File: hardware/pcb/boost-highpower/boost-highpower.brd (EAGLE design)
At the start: 41.1 x 22.3 mm, 28 parts

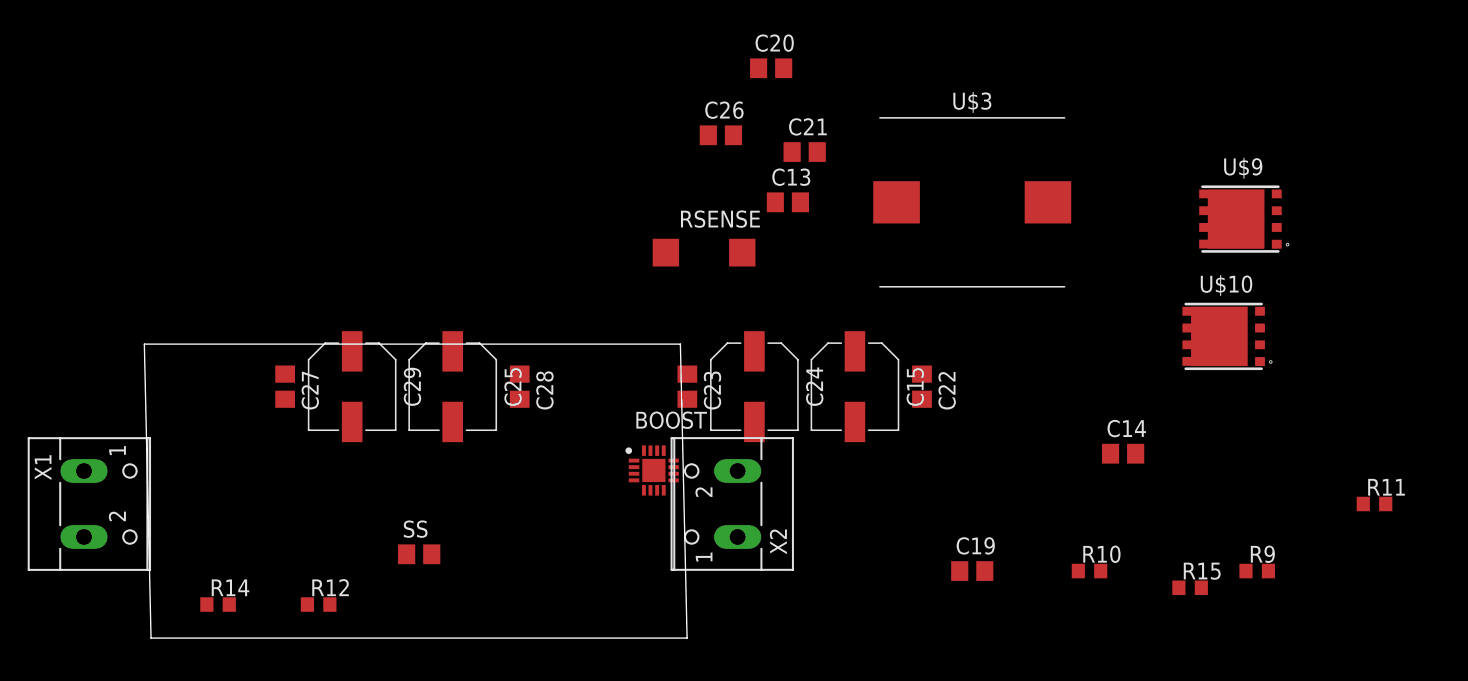
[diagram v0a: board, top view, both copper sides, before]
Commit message: moved some components
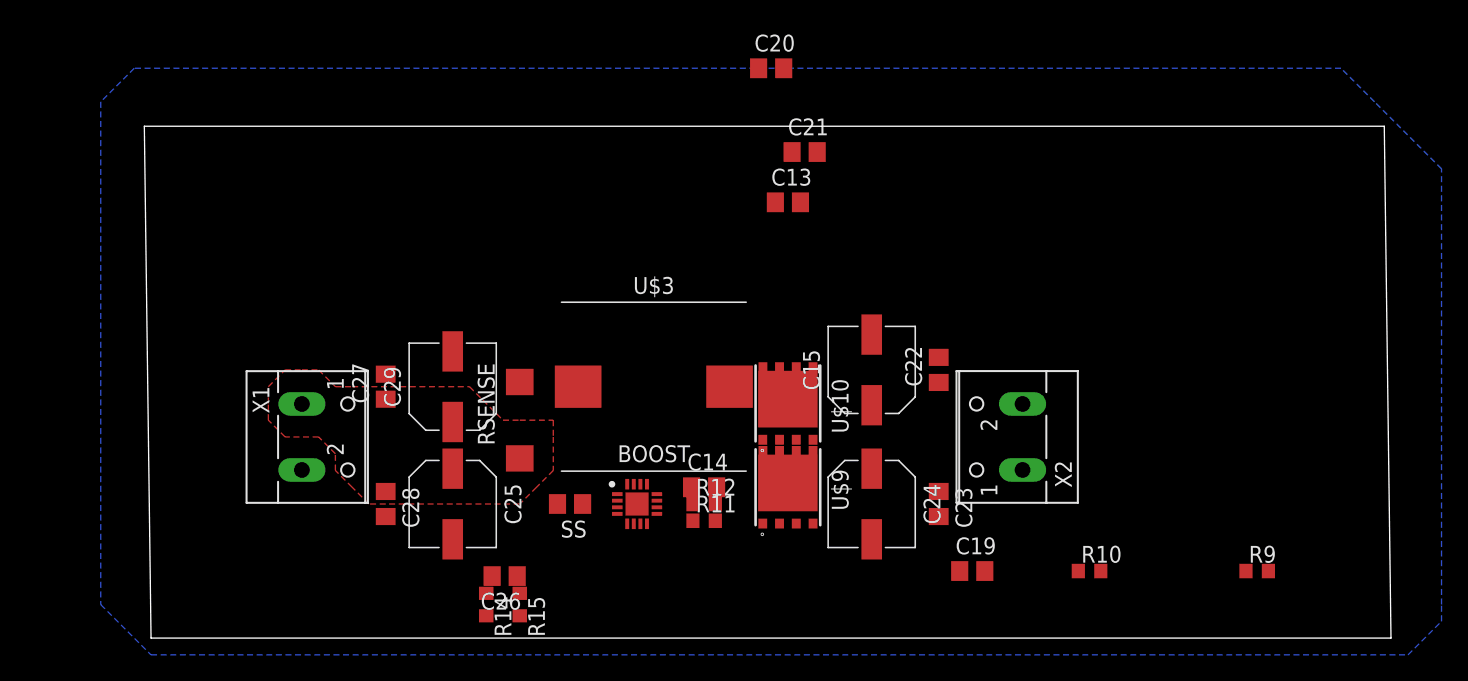
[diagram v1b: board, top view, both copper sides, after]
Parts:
- moved R11 50.8 mm to (41.9, 8.89)
- moved R15 50.8 mm to (27.9, 2.54), turned to 270 degrees
- moved U$9 39.9 mm to (48.3, 11.4), turned to 270 degrees
- moved C26 37.2 mm to (26.8, 4.70), turned to 180 degrees
- moved U$10 33.4 mm to (48.3, 17.8), turned to 270 degrees
- moved C14 31.9 mm to (41.9, 11.4)
- moved R12 30.2 mm to (41.9, 10.2)
- moved U$3 27.9 mm to (38.1, 19.1)
- moved X2 22.2 mm to (64.8, 15.2)
- moved C23 21.0 mm to (59.7, 10.2)
- moved R14 20.3 mm to (25.4, 2.54), turned to 270 degrees
- moved RSENSE 18.9 mm to (27.9, 16.5), turned to 90 degrees
- moved X1 17.3 mm to (12.7, 15.2)
- moved C28 13.5 mm to (17.8, 10.2)
- moved C24 12.6 mm to (54.6, 10.2)
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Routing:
- added copper zone on layer 16, net GND
- added copper zone on layer 1, net VIN
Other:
- board size 41.1 x 22.3 mm -> 94.5 x 38.8 mm
